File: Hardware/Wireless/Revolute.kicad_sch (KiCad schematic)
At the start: 52 parts, among them U1 BQ27441-G1, U2 Button, U2 nrf52833_qfn40, U3 AS5600, U4 AP2112K-3.3, U5 BQ24075RGT, X1 32.768 kHz, X2 32MHZ

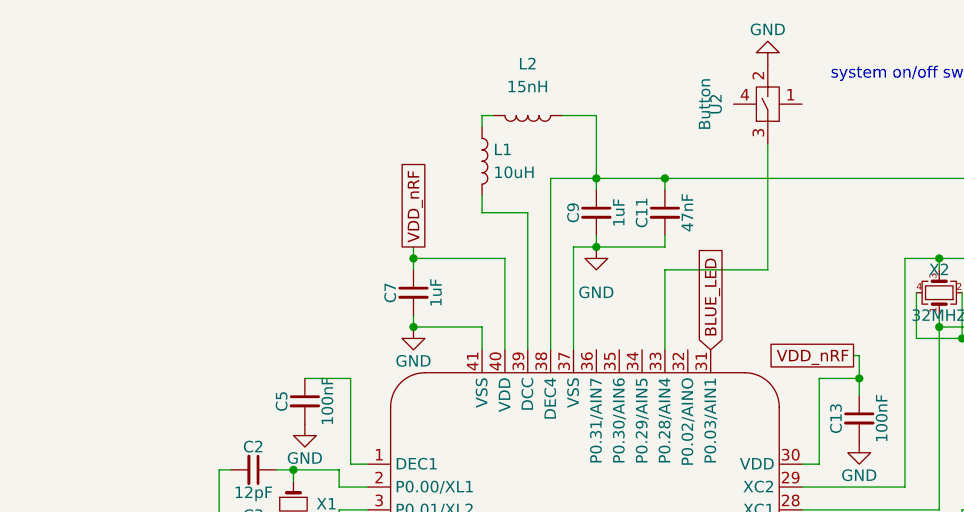
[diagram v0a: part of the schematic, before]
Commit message: implemented 4button design
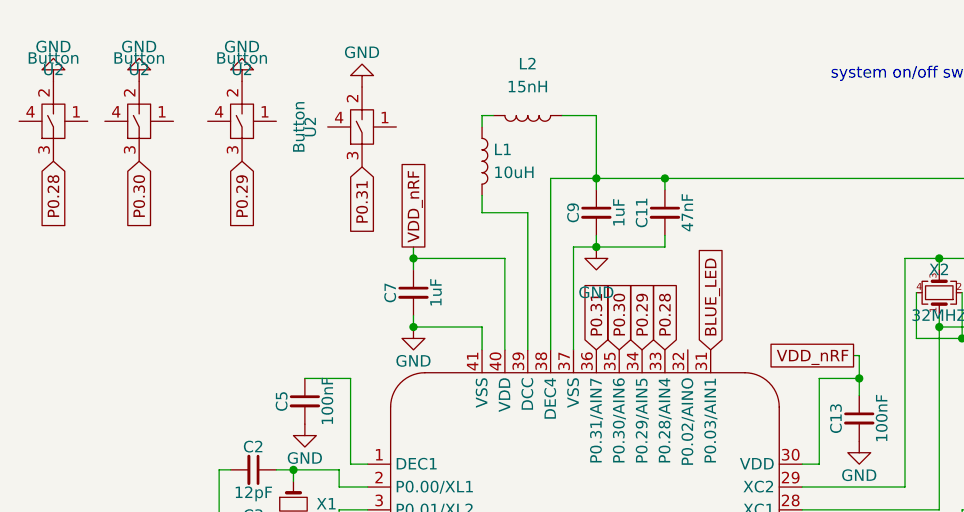
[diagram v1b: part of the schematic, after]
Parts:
- added U2 (x3): Button, Library:SMDButton, symbol Library:Button
- U2: footprint Library:buttoncompliant -> Library:SMDButton
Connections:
- net GND: now also U2.2, U2.2, U2.2
- net P0.28: now reaches U2.33 (P0.28/AIN4)
- net P0.28: now also U2.3; no longer U2.3
- net P0.29: now reaches U2.34 (P0.29/AIN5)
- net P0.29: now also U2.3
- net P0.30: now reaches U2.35 (P0.30/AIN6)
- net P0.30: now also U2.3
- net P0.31: now reaches U2.36 (P0.31/AIN7)
- net P0.31: now also U2.3
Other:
- moved on the sheet: U2
